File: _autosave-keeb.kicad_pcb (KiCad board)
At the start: 2 copper layers, 466.6 x 138.7 mm, 433 parts, among them SW1 SW_Push, SW10 SW_Push, SW100 SW_Push, SW101 SW_Push, SW102 SW_Push, SW103 SW_Push, SW104 SW_Push, SW105 SW_Push, SW11 SW_Push, SW12 SW_Push, SW13 SW_Push, SW14 SW_Push, SW15 SW_Push, SW16 SW_Push, SW17 SW_Push, SW18 SW_Push, SW19 SW_Push, SW2 SW_Push, SW20 SW_Push, SW21 SW_Push, SW22 SW_Push, SW23 SW_Push, SW24 SW_Push, SW25 SW_Push, SW26 SW_Push, SW27 SW_Push, SW28 SW_Push, SW29 SW_Push, SW3 SW_Push, SW30 SW_Push, SW31 SW_Push, SW32 SW_Push, SW33 SW_Push, SW34 SW_Push, SW35 SW_Push, SW36 SW_Push, SW37 SW_Push, SW38 SW_Push, SW39 SW_Push, SW4 SW_Push, SW40 SW_Push, SW41 SW_Push, SW42 SW_Push, SW43 SW_Push, SW44 SW_Push, SW45 SW_Push, SW46 SW_Push, SW47 SW_Push, SW48 SW_Push, SW49 SW_Push, SW5 SW_Push, SW50 SW_Push, SW51 SW_Push, SW52 SW_Push, SW53 SW_Push, SW54 SW_Push, SW55 SW_Push, SW56 SW_Push, SW57 SW_Push, SW58 SW_Push, SW59 SW_Push, SW6 SW_Push, SW60 SW_Push, SW61 SW_Push, SW62 SW_Push, SW63 SW_Push, SW64 SW_Push, SW65 SW_Push, SW66 SW_Push, SW67 SW_Push, SW68 SW_Push, SW69 SW_Push, SW7 SW_Push, SW70 SW_Push, SW71 SW_Push, SW72 SW_Push, SW73 SW_Push, SW74 SW_Push, SW75 SW_Push, SW76 SW_Push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

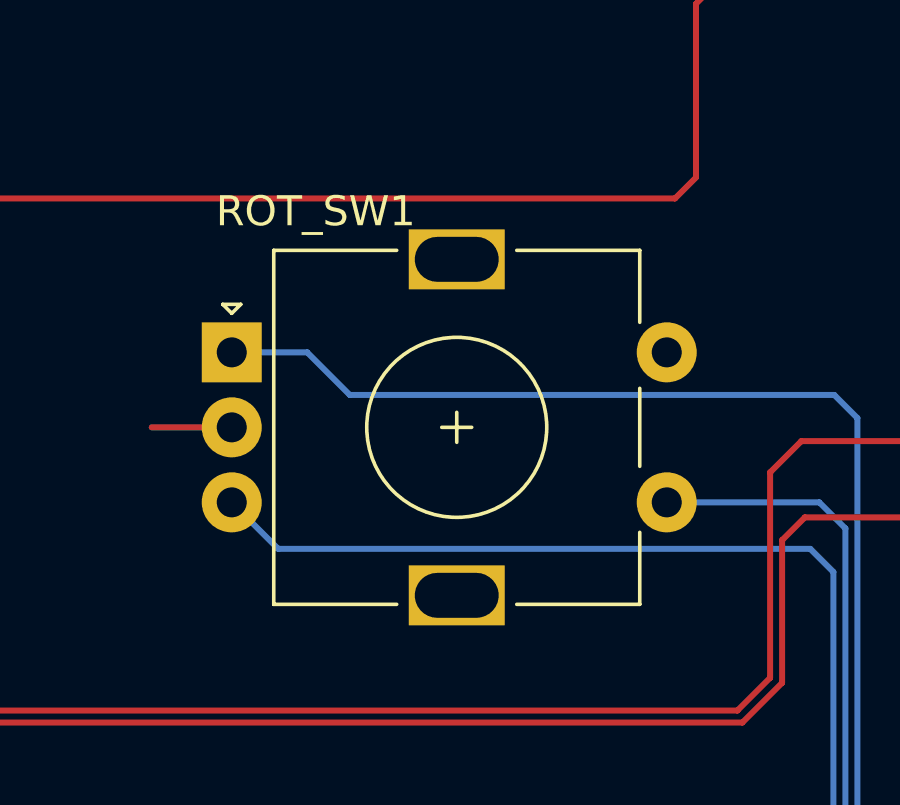
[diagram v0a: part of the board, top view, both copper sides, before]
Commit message: IM FREEEE
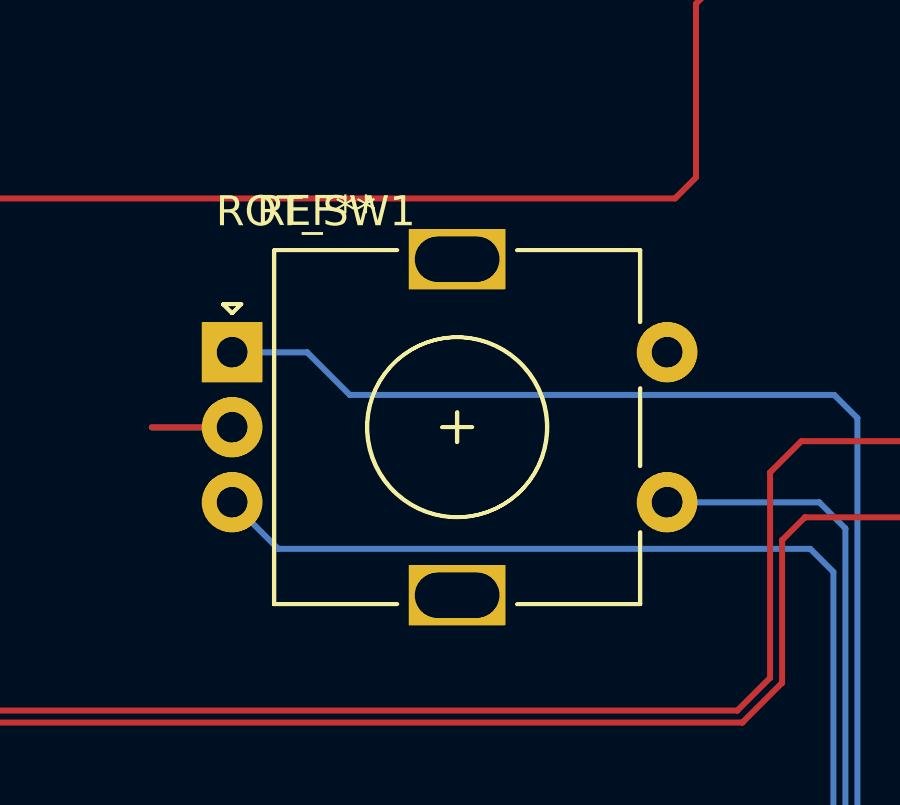
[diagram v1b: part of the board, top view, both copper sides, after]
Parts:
- added REF**: RotaryEncoder_Alps_EC11E-Switch_Vertical_H20mm, Rotary_Encoder:RotaryEncoder_Alps_EC11E-Switch_Vertical_H20mm, F.Cu at (440.4, 35.6)
